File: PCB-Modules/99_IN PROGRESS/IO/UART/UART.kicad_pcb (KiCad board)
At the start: 4 copper layers, 67.6 x 32.8 mm, 32 parts, among them J1 Conn_01x09, J2 Conn_01x08, U1 full-can-crystal, U10 74LS193, U11 74LS193, U12 74LS164, U13 74LS574, U14 74HC245PW,118, U2 74LS193, U3 74LS193, U4 74LS165, U5 74LS165, U6 74HC245PW,118, U7 74LS04, U8 74LS00, U9 74LS00

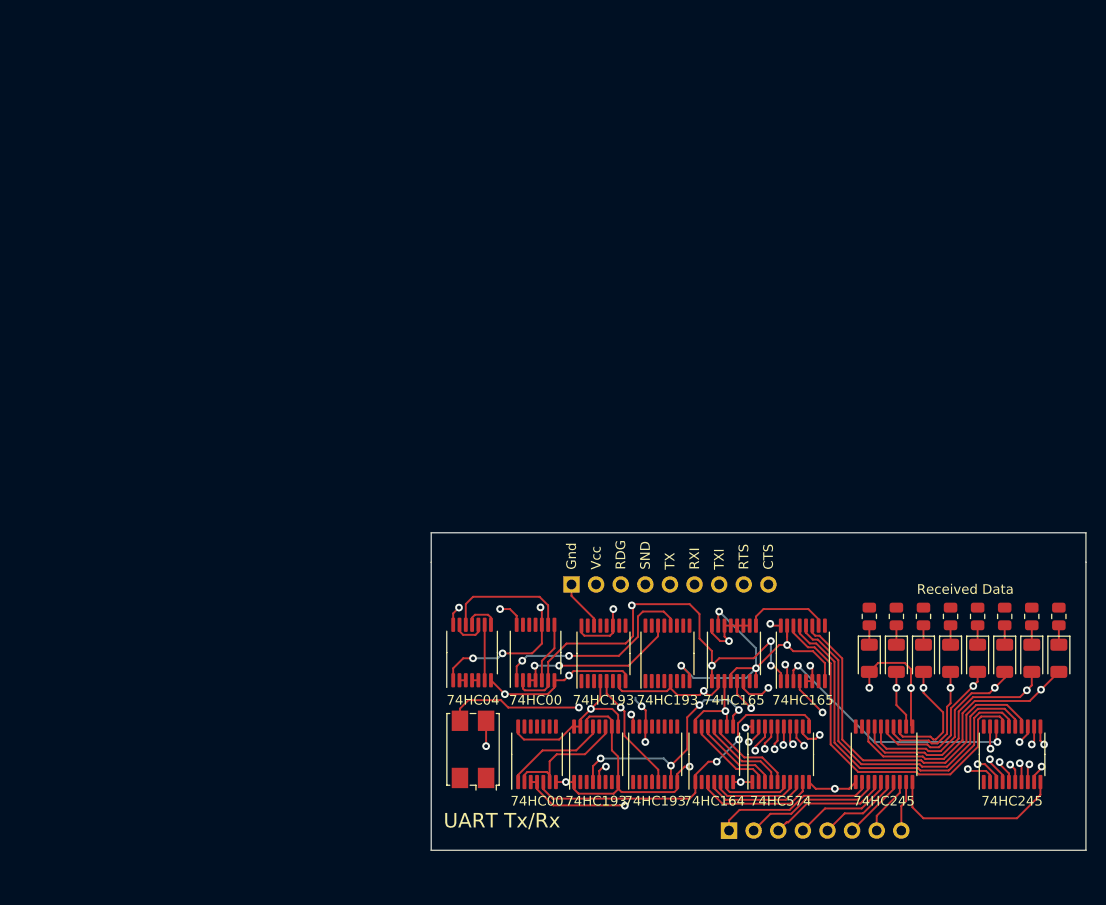
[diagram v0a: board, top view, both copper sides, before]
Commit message: STUPID UPDATE MAJOR SAVE
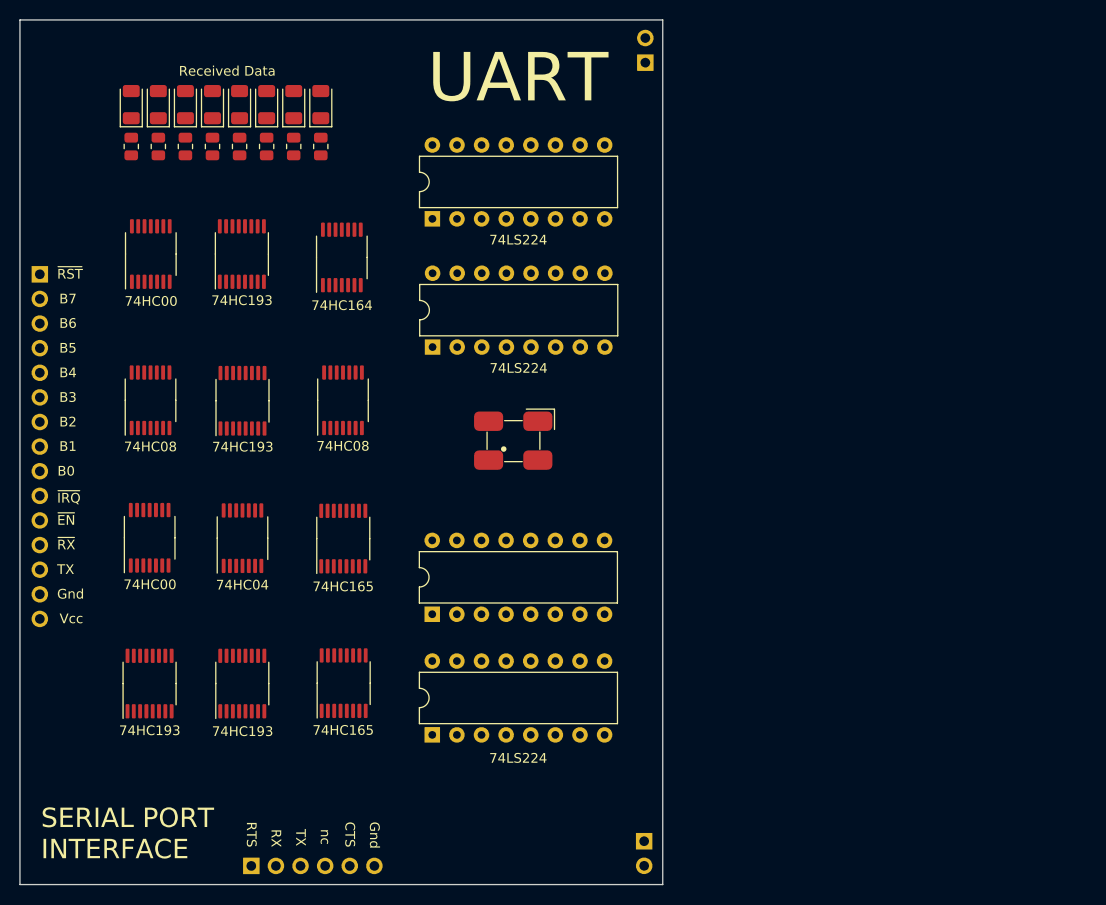
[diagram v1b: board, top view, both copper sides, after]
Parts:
- added J3: Conn_01x02, Connector_PinHeader_2.54mm:PinHeader_1x02_P2.54mm_Vertical, B.Cu at (129.5, 51.3)
- added J4: Conn_01x02, Connector_PinHeader_2.54mm:PinHeader_1x02_P2.54mm_Vertical, B.Cu at (129.4, 131.7)
- added U15: 74LS224, Package_DIP:DIP-16_W7.62mm, F.Cu at (107.6, 120.7)
- added U18: 74LS224, Package_DIP:DIP-16_W7.62mm, F.Cu at (107.5, 108.2)
- added Y1: Crystal_GND24, Stephenv6:CFPS-72 SMD Clock, F.Cu at (116.0, 80.1)
- J1: value Conn_01x09 -> Conn_01x06; footprint Connector_PinHeader_2.54mm:PinHeader_1x09_P2.54mm_Vertical -> Connector_PinHeader_2.54mm:PinHeader_1x06_P2.54mm_Vertical
- J2: value Conn_01x08 -> Conn_01x15; footprint Connector_PinHeader_2.54mm:PinHeader_1x08_P2.54mm_Vertical -> Connector_PinHeader_2.54mm:PinHeader_1x15_P2.54mm_Vertical
- U1: value full-can-crystal -> 74LS193; footprint Crystal:Crystal_SMD_7050-4Pin_7.0x5.0mm -> Package_SO:TSSOP-16_4.4x5mm_P0.65mm
- U10, U11: value 74LS193 -> 74LS165
- U12: value 74LS164 -> 74LS224; footprint Package_SO:TSSOP-14_4.4x5mm_P0.65mm -> Package_DIP:DIP-16_W7.62mm
- U13: value 74LS574 -> 74LS224; footprint Package_SO:TSSOP-20_4.4x6.5mm_P0.65mm -> Package_DIP:DIP-16_W7.62mm
- U14: value 74HC245PW,118 -> 74LS08; footprint Package_SO:TSSOP-20_4.4x6.5mm_P0.65mm -> Package_SO:TSSOP-14_4.4x5mm_P0.65mm
- U4: value 74LS165 -> 74LS193
- U5: value 74LS165 -> 74LS08; footprint Package_SO:TSSOP-16_4.4x5mm_P0.65mm -> Package_SO:TSSOP-14_4.4x5mm_P0.65mm
- U6: value 74HC245PW,118 -> 74LS00; footprint Package_SO:TSSOP-20_4.4x6.5mm_P0.65mm -> Package_SO:TSSOP-14_4.4x5mm_P0.65mm
- U7: value 74LS04 -> 74LS00
- U8: value 74LS00 -> 74LS04
- U9: value 74LS00 -> 74HC164
- moved D1 95.2 mm to (76.5, 55.6), turned to 90 degrees
- moved D2 95.2 mm to (79.3, 55.6), turned to 90 degrees
- moved D3 95.2 mm to (82.1, 55.6), turned to 90 degrees
- moved D4 95.2 mm to (84.9, 55.6), turned to 90 degrees
- moved D5 95.2 mm to (87.7, 55.6), turned to 90 degrees
- moved D6 95.2 mm to (90.5, 55.6), turned to 90 degrees
- moved D7 95.2 mm to (93.3, 55.6), turned to 90 degrees
- moved D8 95.2 mm to (96.0, 55.6), turned to 90 degrees
- moved U6 91.8 mm to (78.4, 100.3)
- moved J2 91.4 mm to (67.1, 73.2), turned to 180 degrees
- moved R2 90.3 mm to (79.3, 60.0), turned to -90 degrees
- moved R4 90.3 mm to (84.9, 60.0), turned to -90 degrees
- moved R5 90.3 mm to (87.7, 60.0), turned to -90 degrees
- moved R7 90.3 mm to (93.3, 60.0), turned to -90 degrees
- moved R1 90.3 mm to (76.5, 60.0), turned to -90 degrees
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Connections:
- D1 pad 2: TXQ7 -> /TX7
- D2 pad 2: TXQ6 -> /TX6
- D3 pad 2: TXQ5 -> /TX5
- D4 pad 2: TXQ4 -> /TX4
- D5 pad 2: TXQ3 -> /TX3
- D6 pad 2: TXQ2 -> /TX2
- D7 pad 2: TXQ1 -> /TX1
- D8 pad 2: TXQ0 -> /TX0
- J1 pad 1: GND -> SER_RTS
- J1 pad 2: VCC -> SER_RX
- J1 pad 3: SEND_DATA -> SER_TX
- J1 pad 4: ~TRANSMIT_DATA_FROM_BUS -> unconnected-(J1-Pad4)
- J1 pad 5: RX_IN_CABLE -> SER_CTS
- J1 pad 6: TX_IN_CABLE -> GND
- J2 pad 1: BUS0 -> ~{RESET_BUFFERS}
- J2 pad 2: BUS1 -> BUS0
- J2 pad 3: BUS2 -> BUS1
- J2 pad 4: BUS3 -> BUS2
- J2 pad 5: BUS4 -> BUS3
- J2 pad 6: BUS5 -> BUS4
- J2 pad 7: BUS6 -> BUS5
- J2 pad 8: BUS7 -> BUS6
- U1 pad 1: Net-(U1-Pad1) -> GND
- U1 pad 2: GND -> unconnected-(U1-Pad2)
- U1 pad 3: Net-(U1-Pad3) -> unconnected-(U1-Pad3)
- U1 pad 4: VCC -> Net-(U1-Pad4)
- U10 pad 1: GND -> /TX_START
- U10 pad 10: GND -> Net-(U10-Pad10)
- U10 pad 11: Net-(U10-Pad11) -> RX5
- U10 pad 12: Net-(U10-Pad12) -> RX4
- U10 pad 13: Net-(U10-Pad13) -> RX3
- U10 pad 14: GND -> RX2
- U10 pad 15: VCC -> GND
- U10 pad 2: Net-(U10-Pad2) -> /TX_CLOCK
- U10 pad 3: Net-(U10-Pad3) -> RX1
- U10 pad 4: Net-(U10-Pad4) -> RX0
- U10 pad 5: VCC -> GND
- U10 pad 6: Net-(U10-Pad6) -> VCC
- U10 pad 7: Net-(U10-Pad7) -> unconnected-(U10-Pad7)
- U10 pad 9: VCC -> SER_RX
- U11 pad 1: Net-(U11-Pad1) -> /TX_START
- U11 pad 10: Net-(U11-Pad10) -> VCC
- U11 pad 12: Net-(U11-Pad12) -> VCC
- U11 pad 13: Net-(U11-Pad13) -> VCC
- U11 pad 14: RECEIVING_DATA -> VCC
- U11 pad 15: Net-(U11-Pad15) -> GND
- U11 pad 2: Net-(U11-Pad2) -> /TX_CLOCK
- U11 pad 3: Net-(U11-Pad3) -> VCC
- U11 pad 5: Net-(U1-Pad3) -> RX7
- U11 pad 6: Net-(U11-Pad6) -> RX6
- U11 pad 7: Net-(U10-Pad4) -> unconnected-(U11-Pad7)
- U11 pad 9: Net-(U11-Pad9) -> Net-(U10-Pad10)
- U12 pad 1: TX_IN_CABLE -> /READ
- U12 pad 10: TX3 -> BUS3
- U12 pad 11: TX2 -> BUS2
- U12 pad 12: TX1 -> BUS1
- U12 pad 13: TX0 -> BUS0
- U12 pad 14: VCC -> Net-(U12-Pad14)
- U12 pad 2: VCC -> Net-(U12-Pad2)
- U12 pad 3: TX7 -> /WRITE
- U12 pad 4: TX6 -> /TX0
- U12 pad 5: TX5 -> /TX1
- U12 pad 6: TX4 -> /TX2
- U12 pad 7: GND -> /TX3
- U12 pad 8: Net-(U10-Pad4) -> GND
- U12 pad 9: VCC -> ~{RESET_BUFFERS}
- U13 pad 1: GND -> /READ
- U13 pad 10: GND -> BUS7
- U13 pad 11: TX_IN_CABLE -> BUS6
- U13 pad 12: TXQ7 -> BUS5
- U13 pad 13: TXQ6 -> BUS4
- U13 pad 14: TXQ5 -> Net-(U13-Pad14)
- U13 pad 15: TXQ4 -> /READ
- U13 pad 16: TXQ3 -> VCC
- U13 pad 2: TX0 -> Net-(U13-Pad2)
- U13 pad 3: TX1 -> /WRITE
- U13 pad 4: TX2 -> /TX4
- U13 pad 5: TX3 -> /TX5
- U13 pad 6: TX4 -> /TX6
- U13 pad 7: TX5 -> /TX7
- U13 pad 8: TX6 -> GND
- U13 pad 9: TX7 -> ~{RESET_BUFFERS}
- U14 pad 1: GND -> EN
- U14 pad 10: GND -> Net-(U13-Pad14)
- U14 pad 11: TXQ7 -> unconnected-(U14-Pad11)
- U14 pad 12: TXQ6 -> GND
- U14 pad 13: TXQ5 -> GND
- U14 pad 14: TXQ4 -> VCC
- U14 pad 2: BUS0 -> RECEIVE_BYTE
- U14 pad 3: BUS1 -> /READ
- U14 pad 4: BUS2 -> Net-(U12-Pad2)
- U14 pad 5: BUS3 -> Net-(U13-Pad2)
- U14 pad 6: BUS4 -> SER_CTS
- U14 pad 7: BUS5 -> GND
- U14 pad 8: BUS6 -> Net-(U8-Pad1)
- U14 pad 9: BUS7 -> Net-(U12-Pad14)
- U2 pad 1: Net-(U2-Pad1) -> GND
- U2 pad 10: Net-(U2-Pad10) -> GND
- U2 pad 12: Net-(U2-Pad12) -> unconnected-(U2-Pad12)
- U2 pad 13: Net-(U2-Pad13) -> unconnected-(U2-Pad13)
- U2 pad 15: Net-(U2-Pad15) -> GND
- U2 pad 2: Net-(U2-Pad2) -> unconnected-(U2-Pad2)
- U2 pad 3: Net-(U2-Pad3) -> unconnected-(U2-Pad3)
- U2 pad 5: Net-(U1-Pad3) -> UART_CLOCK
- U2 pad 6: Net-(U2-Pad6) -> unconnected-(U2-Pad6)
- U2 pad 7: CLK -> /TX_CLOCK
- U2 pad 9: Net-(U2-Pad9) -> GND
- U3 pad 1: Net-(U3-Pad1) -> GND
- U3 pad 10: Net-(U3-Pad10) -> GND
- U3 pad 12: CO -> unconnected-(U3-Pad12)
- U3 pad 13: Net-(U3-Pad13) -> unconnected-(U3-Pad13)
- U3 pad 14: CLR -> /WRITE
- U3 pad 15: Net-(U3-Pad15) -> GND
- U3 pad 2: Net-(U3-Pad2) -> unconnected-(U3-Pad2)
- U3 pad 3: Net-(U3-Pad3) -> unconnected-(U3-Pad3)
- U3 pad 5: CLK -> UART_CLOCK
- U3 pad 6: Net-(U3-Pad6) -> unconnected-(U3-Pad6)
- U3 pad 7: Net-(U3-Pad7) -> Net-(U1-Pad4)
- U3 pad 9: Net-(U3-Pad9) -> GND
- U4 pad 1: SH~LD -> GND
- U4 pad 10: Net-(U4-Pad10) -> VCC
- U4 pad 11: RX4 -> /TX_START
- U4 pad 12: RX3 -> Net-(U4-Pad12)
- U4 pad 13: RX2 -> unconnected-(U4-Pad13)
- U4 pad 14: RX1 -> GND
- U4 pad 15: GND -> VCC
- U4 pad 2: CLK -> unconnected-(U4-Pad2)
- U4 pad 3: RX0 -> unconnected-(U4-Pad3)
- U4 pad 4: RX7 -> VCC
- U4 pad 5: VCC -> /TX_CLOCK
- U4 pad 6: VCC -> unconnected-(U4-Pad6)
- U4 pad 7: Net-(U4-Pad7) -> unconnected-(U4-Pad7)
- U4 pad 9: RX_IN_CABLE -> GND
- U5 pad 1: SH~LD -> TRANSMIT_BYTE
- U5 pad 10: VCC -> Net-(U18-Pad14)
- U5 pad 11: VCC -> unconnected-(U5-Pad11)
- U5 pad 12: VCC -> GND
- U5 pad 13: VCC -> GND
- U5 pad 2: CLK -> EN
- U5 pad 3: VCC -> TRANSMIT_BYTE
- U5 pad 4: GND -> Net-(U15-Pad2)
- U5 pad 5: RX6 -> Net-(U5-Pad5)
- U5 pad 6: RX5 -> unconnected-(U5-Pad6)
- U5 pad 7: Net-(U5-Pad7) -> GND
- U5 pad 8: GND -> Net-(U5-Pad8)
- U5 pad 9: Net-(U4-Pad10) -> Net-(U15-Pad14)
- U6 pad 1: VCC -> TF_DATA_READ
- U6 pad 10: GND -> /TX_CLOCK
- U6 pad 11: RX7 -> unconnected-(U6-Pad11)
- U6 pad 12: RX6 -> GND
- U6 pad 13: RX5 -> GND
- U6 pad 14: RX4 -> VCC
- U6 pad 2: BUS0 -> Net-(U6-Pad2)
- U6 pad 3: BUS1 -> /TX_START
- U6 pad 4: BUS2 -> Net-(U4-Pad12)
- U6 pad 5: BUS3 -> /TX_START
- U6 pad 6: BUS4 -> TF_DATA_READ
- U6 pad 7: BUS5 -> GND
- U6 pad 8: BUS6 -> Net-(U6-Pad2)
- U6 pad 9: BUS7 -> SER_RTS
- U7 pad 1: SEND_DATA -> Net-(U1-Pad13)
- U7 pad 10: Net-(U7-Pad10) -> GND
- U7 pad 11: Net-(U7-Pad11) -> unconnected-(U7-Pad11)
- U7 pad 12: Net-(U7-Pad12) -> GND
- U7 pad 13: Net-(U7-Pad10) -> GND
- U7 pad 2: Net-(U7-Pad2) -> Net-(U1-Pad11)
- U7 pad 3: Net-(U7-Pad2) -> /WRITE
- U7 pad 4: Net-(U7-Pad4) -> /WRITE
- U7 pad 5: Net-(U7-Pad4) -> SER_TX
- U7 pad 6: Net-(U7-Pad6) -> Net-(U1-Pad11)
- U7 pad 8: Net-(U7-Pad11) -> unconnected-(U7-Pad8)
- U7 pad 9: Net-(U7-Pad6) -> GND
- U8 pad 1: CO -> Net-(U8-Pad1)
- U8 pad 10: SEND_DATA -> SER_RTS
- U8 pad 11: (no net) -> Net-(U5-Pad8)
- U8 pad 12: (no net) -> unconnected-(U8-Pad12)
- U8 pad 13: (no net) -> GND
- U8 pad 2: SH~LD -> ~{RX_IRQ}
- U8 pad 3: CLR -> ~{RECEIVE_BYTE}
- U8 pad 4: CLR -> RECEIVE_BYTE
- U8 pad 5: Net-(U8-Pad5) -> ~{EN}
- U8 pad 6: SH~LD -> EN
- U8 pad 8: Net-(U8-Pad5) -> TRANSMIT_BYTE
- U8 pad 9: Net-(U7-Pad12) -> ~{TRANSMIT_BYTE}
- U9 pad 1: Net-(U10-Pad13) -> SER_TX
- U9 pad 10: (no net) -> /TX4
- U9 pad 11: (no net) -> /TX5
- U9 pad 12: (no net) -> /TX6
- U9 pad 13: (no net) -> /TX7
- U9 pad 2: Net-(U10-Pad11) -> VCC
- U9 pad 3: RECEIVING_DATA -> /TX0
- U9 pad 4: RECEIVING_DATA -> /TX1
- U9 pad 5: TX_IN_CABLE -> /TX2
- U9 pad 6: Net-(U10-Pad11) -> /TX3
- U9 pad 8: (no net) -> Net-(U1-Pad4)
- U9 pad 9: (no net) -> VCC
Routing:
- net GND: track 174.3 -> 0.00 mm, vias 11 -> 0
- net TXQ0: track 65.5 -> 0.00 mm, vias 2 -> 0
- net VCC: track 61.1 -> 0.00 mm, vias 11 -> 0
- net TXQ1: track 59.5 -> 0.00 mm, vias 2 -> 0
- net TXQ2: track 50.5 -> 0.00 mm, vias 2 -> 0
- net BUS0: track 47.4 -> 0.00 mm, vias 1 -> 0
- net SH~LD: track 46.3 -> 0.00 mm, vias 4 -> 0
- net BUS1: track 43.7 -> 0.00 mm, vias 1 -> 0
- net TXQ3: track 42.8 -> 0.00 mm, vias 2 -> 0
- net BUS2: track 40.6 -> 0.00 mm, vias 1 -> 0
- net RX2: track 38.3 -> 0.00 mm
- net RX1: track 38.2 -> 0.00 mm
- net RX3: track 38.2 -> 0.00 mm
- net RX4: track 38.2 -> 0.00 mm
- net RX6: track 37.6 -> 0.00 mm, vias 2 -> 0
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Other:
- board size 67.6 x 32.8 mm -> 66.3 x 89.2 mm
- net class Default removed
- board text added: "B0"
- board text added: "B1"
- board text added: "B2"
- board text added: "B3"
- board text added: "B4"
- board text added: "B5"
- board text added: "B6"
- board text added: "B7"
- board text added: "RX"
- board text added: "SERIAL PORT INTERFACE"
- board text added: "UART"
- board text added: "nc"
- board text added: "~{EN}"
- board text added: "~{IRQ}"
- board text added: "~{RST}"
- board text added: "~{RX}"
- board text removed: "RDG"
- board text removed: "RXI"
- board text removed: "SND"
- board text removed: "TXI"
- board text removed: "UART Tx/Rx"
